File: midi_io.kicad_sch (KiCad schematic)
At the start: 7 parts

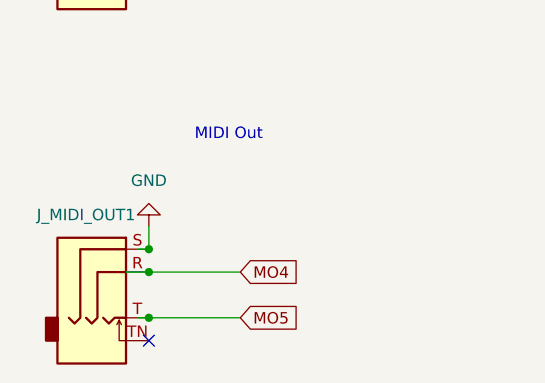
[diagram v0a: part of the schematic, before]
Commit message: Solve all warnings
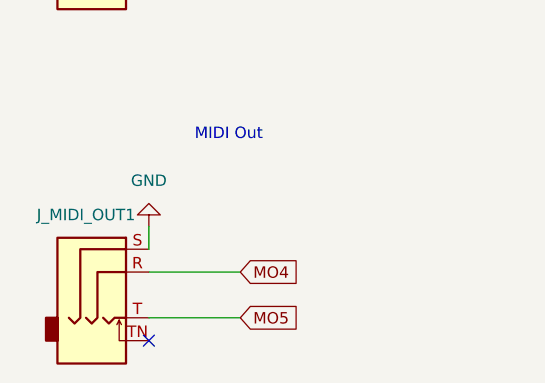
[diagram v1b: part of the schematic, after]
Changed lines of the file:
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@@
-		(color 0 0 0 0)
-	)
-	(junction
-		(at 58.42 87.63)
-		(diameter 0)
-		(color 0 0 0 0)
-	)
-	(junction
-		(at 58.42 95.25)
-		(diameter 0)
-		(color 0 0 0 0)
-	)
-	(junction
-		(at 58.42 90.17)
-		(diameter 0)
 		(color 0 0 0 0)
 	)
@@
 		(pts
 			(xy 58.42 55.88) (xy 73.66 55.88)
-		)
-		(stroke
-			(width 0)
-			(type default)
-		)
-	)
-	(wire
-		(pts
-			(xy 57.15 95.25) (xy 58.42 95.25)
 		)
 		(stroke
@@
 	(wire
 		(pts
-			(xy 58.42 90.17) (xy 68.58 90.17)
-		)
-		(stroke
-			(width 0)
-			(type default)
-		)
-	)
-	(wire
-		(pts
 			(xy 58.42 50.8) (xy 64.77 50.8)
 		)
@@
 	(wire
 		(pts
-			(xy 57.15 87.63) (xy 58.42 87.63)
+			(xy 105.41 49.53) (xy 93.98 49.53)
 		)
 		(stroke
@@
 	(wire
 		(pts
-			(xy 105.41 49.53) (xy 93.98 49.53)
+			(xy 58.42 85.09) (xy 58.42 87.63)
 		)
 		(stroke
@@
 	(wire
 		(pts
-			(xy 64.77 50.8) (xy 64.77 48.26)
+			(xy 58.42 90.17) (xy 68.58 90.17)
 		)
 		(stroke
@@
 	(wire
 		(pts
-			(xy 58.42 85.09) (xy 58.42 87.63)
+			(xy 64.77 50.8) (xy 64.77 48.26)
 		)
 		(stroke
@@
 		)
 		(stroke
-			(width 0)
-			(type default)
-		)
-	)
-	(wire
-		(pts
-			(xy 55.88 90.17) (xy 58.42 90.17)
-		)
-		(stroke
